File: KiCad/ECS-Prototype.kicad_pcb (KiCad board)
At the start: 2 copper layers, 192.1 x 149.8 mm, 53 parts, among them J1 Connector1, J3 FC68131, J4 FC68131, J5 FC68131, Q1 PN2222A, T1 VB_05-1-12, T2 VB_05-1-12, T3 VB_05-1-12, U3 LT1498IN8, U4 MCP602T, U5 MCP602T, U6 MCP602T

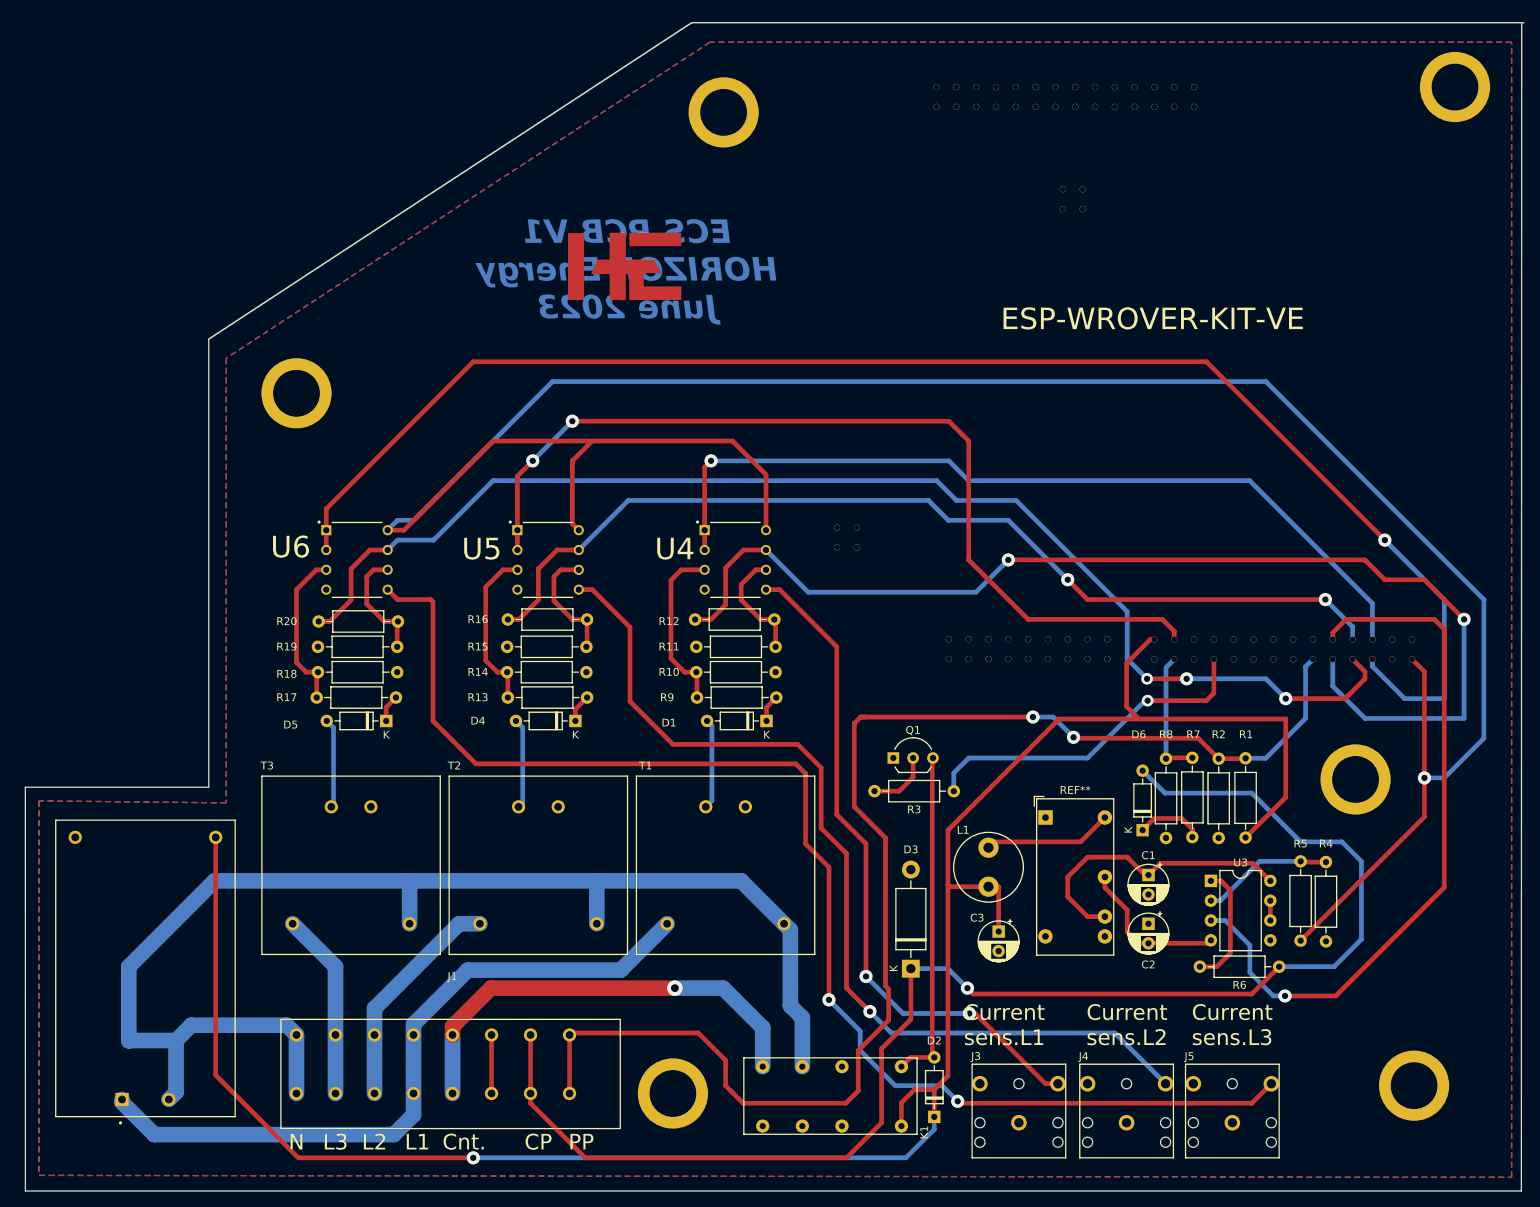
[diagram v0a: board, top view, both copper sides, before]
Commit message: modifications for pcb design: version 3
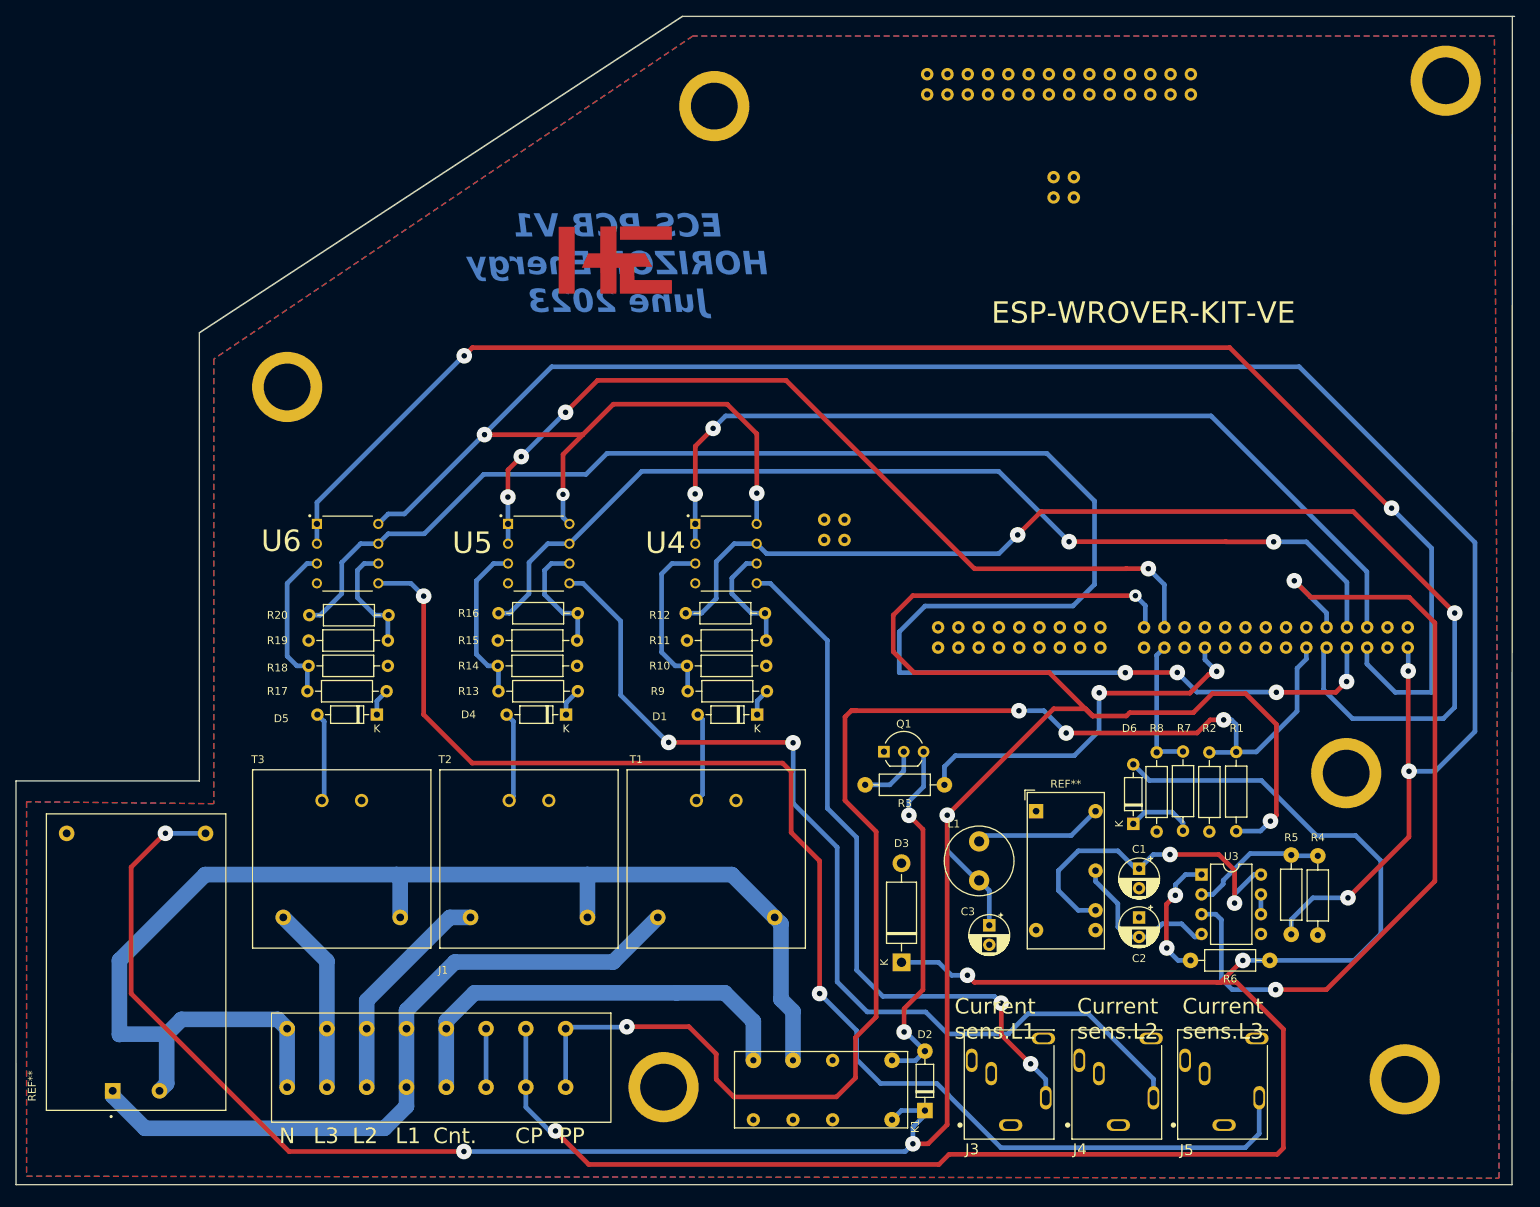
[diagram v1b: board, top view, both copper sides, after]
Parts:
- J3, J4, J5: value FC68131 -> SJ1-3515N; footprint DehneEVSEFootPrints:CLIFF_FC68131 -> ECS-PrototypeFootPrints:CUI_SJ1-3515N
- moved Ref** 1.91 mm to (310.8, 140.9)
- moved ? 1.45 mm to (210.1, 190.4)
- moved ? 1.45 mm to (310.3, 61.4)
- moved C1 1.45 mm to (271.0, 162.4)
- moved C2 1.45 mm to (271.0, 168.7)
- moved C3 1.45 mm to (251.8, 169.7)
- moved D1 1.45 mm to (222.1, 142.7)
- moved D2 1.45 mm to (243.6, 193.4)
- moved D3 1.45 mm to (240.6, 174.4)
- moved D4 1.45 mm to (197.6, 142.7)
- moved D5 1.45 mm to (173.3, 142.7)
- moved D6 1.45 mm to (270.3, 156.7)
- moved G*** 1.45 mm to (203.8, 84.2)
- moved J1 1.45 mm to (159.8, 170.9)
- moved L1 1.45 mm to (250.5, 158.9)
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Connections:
- J3 pad 2: Net-(J3-Pad2) -> CUR_SENS_L1
- J3 pad 5: CUR_SENS_L1 -> (no net)
- J4 pad 2: Net-(J4-Pad2) -> CUR_SENS_L2
- J4 pad 5: CUR_SENS_L2 -> (no net)
- J5 pad 2: Net-(J5-Pad2) -> CUR_SENS_L3
- J5 pad 5: CUR_SENS_L3 -> (no net)
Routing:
- net +5V: track 267.2 -> 348.0 mm, vias 1 -> 6
- net CP: track 184.7 -> 248.7 mm, vias 1 -> 3
- net CURRENT_SENS_L3_READ: track 163.4 -> 220.9 mm, vias 3 -> 4
- net PWM: track 91.2 -> 105.4 mm, vias 1 -> 2
- net VOLTAGE_SENS_L1_READ: track 108.7 -> 115.9 mm, vias 1 -> 2
- net CUR_SENS_L3: track 167.2 -> 173.9 mm
- net +12VDC: track 37.9 -> 44.3 mm, vias 0 -> 2
- net /PP: track 171.9 -> 178.1 mm, vias 2 -> 4
- net DC_RELAY: track 44.2 -> 49.2 mm, vias 1 -> 2
- net CURRENT_SENS_L2_READ: track 125.4 -> 130.3 mm
- net CUR_SENS_L1: track 86.2 -> 90.7 mm
- net +3V3: track 305.7 -> 301.4 mm, vias 1 -> 6
- net CUR_SENS_L2: track 121.7 -> 126.0 mm, vias 1 -> 2
- net Net-(D2-Pad2): track 43.2 -> 47.3 mm, vias 0 -> 2
- net VOLTAGE_SENS_L3_READ: track 193.6 -> 197.5 mm, vias 1 -> 2
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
